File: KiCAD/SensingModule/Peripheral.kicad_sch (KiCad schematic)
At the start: 7 parts, among them J3 DF51-2P-2DS, U10 BME280

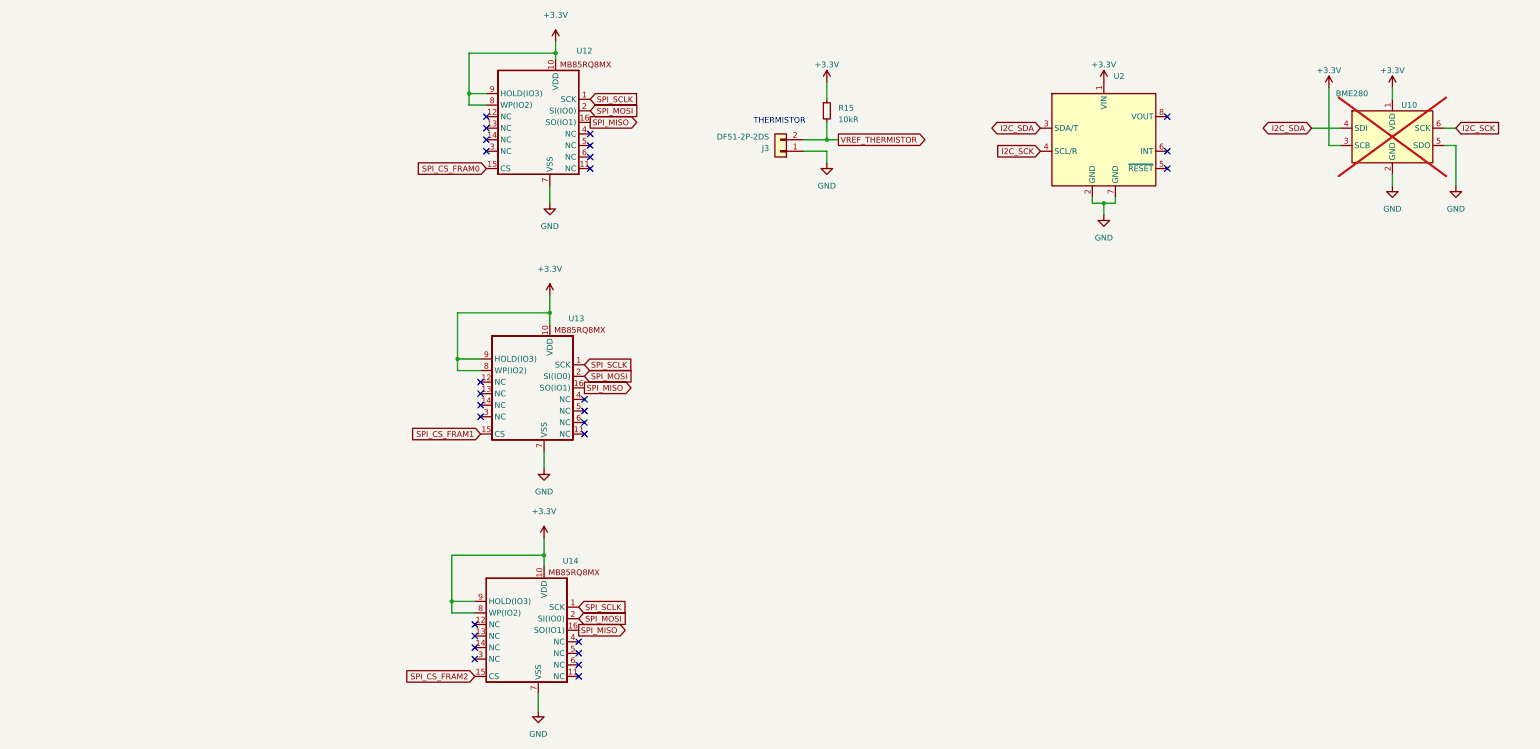
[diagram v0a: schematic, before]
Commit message: きれいに配線できるようになった．
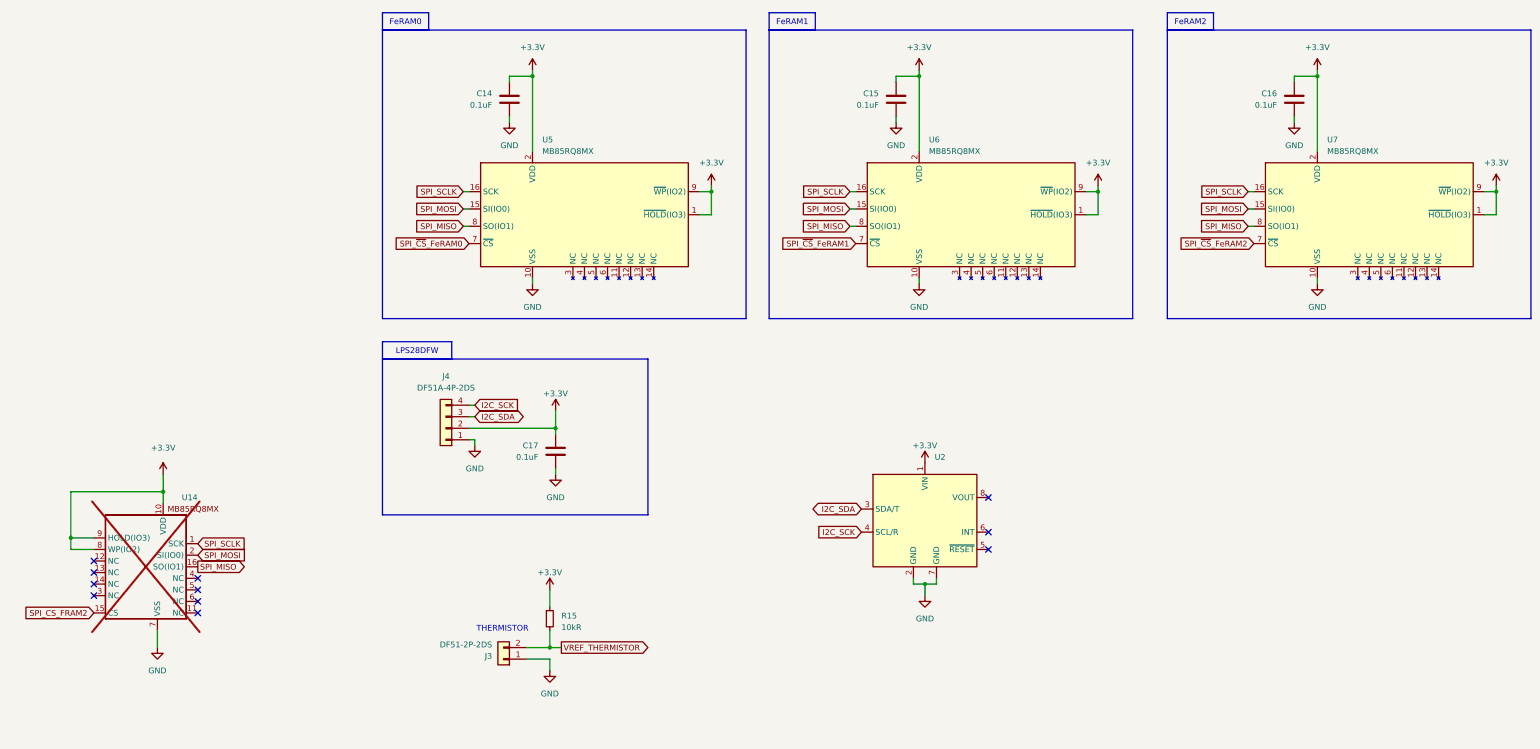
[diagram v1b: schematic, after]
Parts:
- removed U10: BME280, Akizuki_BME280_Module:BME280, symbol Akizuki_BME280_Module:BME280
- removed U12, U13: ~, Package_SO:SOIC-16W_7.5x10.3mm_P1.27mm, symbol MB85RQ8MX_sym:MB85RQMX
- added C14, C15, C16, C17: 0.1uF, Capacitor_SMD:C_0603_1608Metric_Pad1.08x0.95mm_HandSolder, symbol Device:C
- added J4: DF51A-4P-2DS, TSRP_Connector_Hirose:DF51A-4P-2DS, symbol Connector_Generic:Conn_01x04
- added U5, U6, U7: MB85RQ8MX, Package_SO:SOIC-16W_7.5x10.3mm_P1.27mm, symbol TSRP_IC:MB85RQ8MX
- U14: now not fitted; now left out of the parts list
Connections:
- net +3.3V: now also C14.1, C15.1, C16.1, C17.1, J4.2 (Pin_2), U5.1 (~{HOLD}(IO3)), U5.2 (VDD), U5.9 (~{WP}(IO2)), U6.1 (~{HOLD}(IO3)), U6.2 (VDD), U6.9 (~{WP}(IO2)), U7.1 (~{HOLD}(IO3)), U7.2 (VDD), U7.9 (~{WP}(IO2))
- net GND: now also C14.2, C15.2, C16.2, C17.2, J4.1 (Pin_1), U5.10 (VSS), U6.10 (VSS), U7.10 (VSS)
- net I2C_SCK: now also J4.4 (Pin_4)
- net I2C_SDA: now also J4.3 (Pin_3)
- net SPI_MISO: now also U5.8 (SO(IO1)), U6.8 (SO(IO1)), U7.8 (SO(IO1))
- net SPI_MOSI: now also U5.15 (SI(IO0)), U6.15 (SI(IO0)), U7.15 (SI(IO0))
- net SPI_SCLK: now also U5.16 (SCK), U6.16 (SCK), U7.16 (SCK)
- new net SPI_~{CS}_FeRAM0: U5.7 (~{CS})
- new net SPI_~{CS}_FeRAM1: U6.7 (~{CS})
- new net SPI_~{CS}_FeRAM2: U7.7 (~{CS})
- no-connect marks 27 -> 11
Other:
- moved on the sheet: J3, R15, U2
